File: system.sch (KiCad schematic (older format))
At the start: 38 parts, among them IC1 OSD335x, IC3 NAND_4GB, U8 SN74LVC1G06DCK, U9 74LVC1G07DCK, Y1 24MHz, Y2 32.768kHz

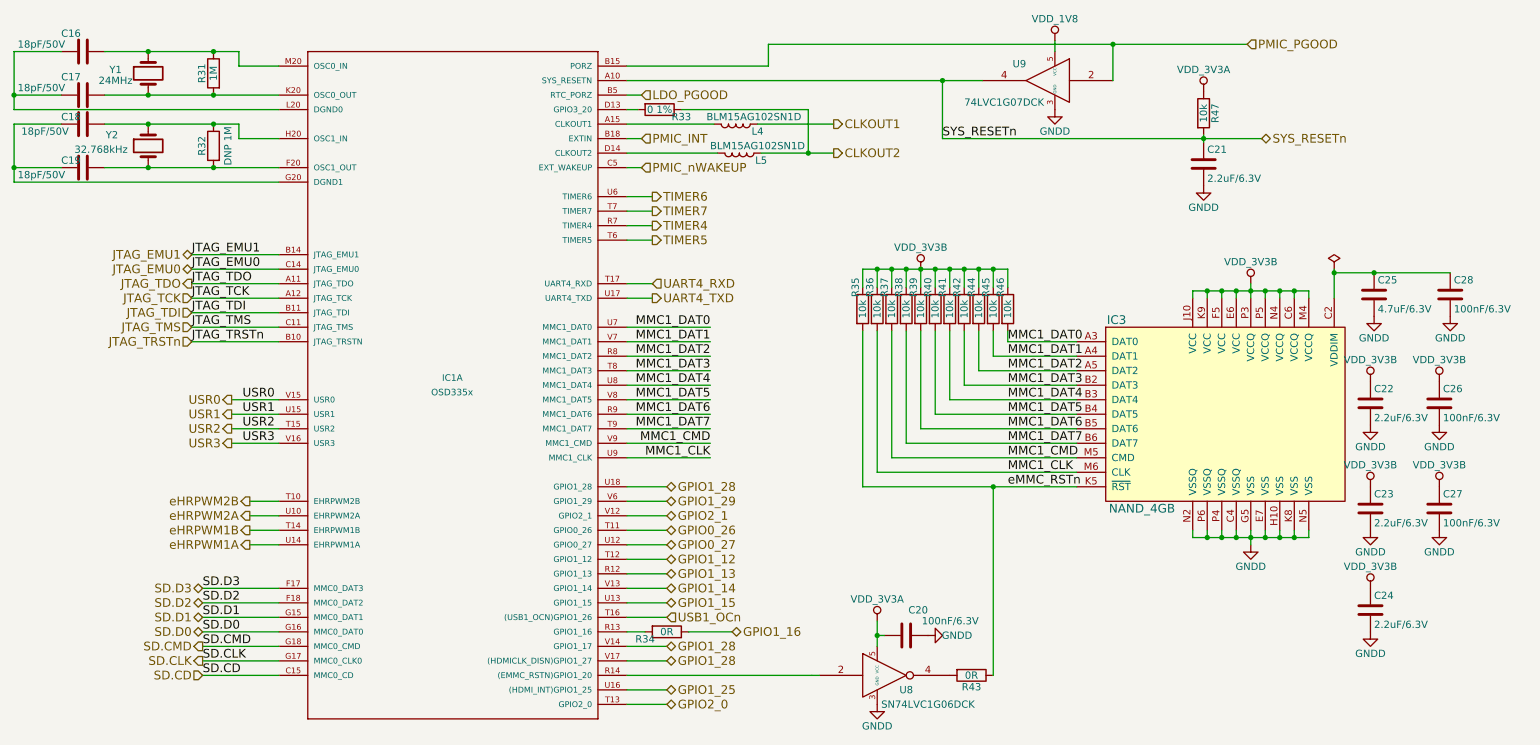
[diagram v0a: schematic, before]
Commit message: wip erc
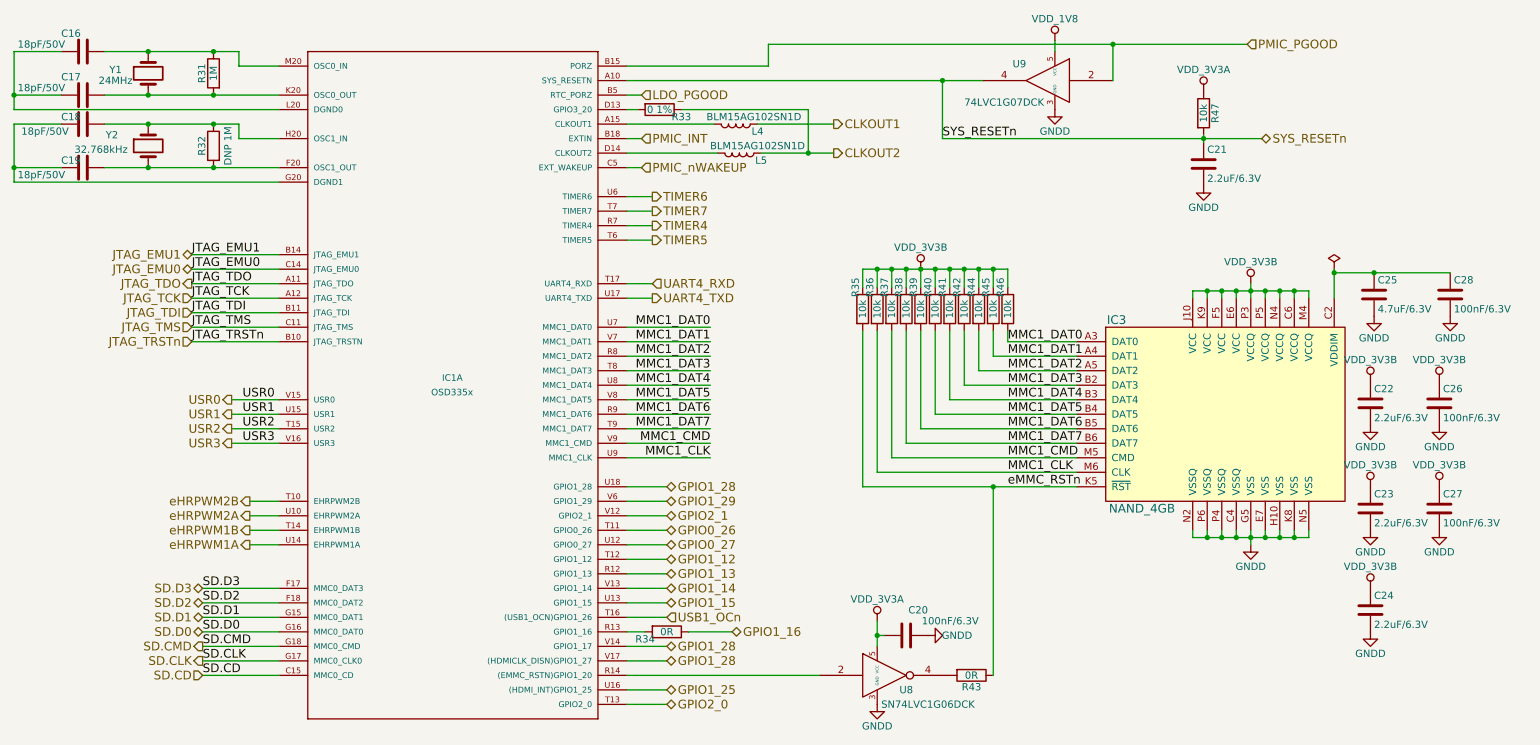
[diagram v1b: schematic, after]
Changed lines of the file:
@@
 $EndComp
 Wire Wire Line
-	1375 775  1675 775
-Wire Wire Line
-	1675 775  2125 775
-Wire Wire Line
-	2125 775  2300 775
-Wire Wire Line
-	1375 1075 1675 1075
-Wire Wire Line
-	1675 1075 2125 1075
-Wire Wire Line
-	2125 1075 2575 1075
+	1375 775  2300 775
+Wire Wire Line
+	1375 1075 2575 1075
 $Comp
 L R R31
@@
 	1075 775  750  775
 Wire Wire Line
-	750  775  750  1075
-Wire Wire Line
-	750  1075 750  1175
+	750  775  750  1175
 Wire Wire Line
 	750  1075 1075 1075
@@
 $EndComp
 Wire Wire Line
-	5950 725  8325 725
-Wire Wire Line
-	8325 725  9250 725
+	5950 725  9250 725
 Text HLabel 9250 725  2    60   Input ~ 0
 PMIC_PGOOD
@@
 $EndComp
 Wire Wire Line
-	4975 975  7150 975
-Wire Wire Line
-	7150 975  7425 975
+	4975 975  7425 975
 $Comp
 L GNDD #PWR75
@@
 Connection ~ 8325 725
 Wire Wire Line
-	7150 1375 8950 1375
-Wire Wire Line
-	8950 1375 9350 1375
+	7150 1375 9350 1375
 Wire Wire Line
 	7150 1375 7150 975
@@
 $EndComp
 Wire Wire Line
-	8950 1350 8950 1375
-Wire Wire Line
-	8950 1375 8950 1400
+	8950 1350 8950 1400
 Connection ~ 8950 1375
 $Comp
@@
 CLKOUT2
 Wire Wire Line
-	5900 1475 6225 1475
-Wire Wire Line
-	6225 1475 6400 1475
+	5900 1475 6400 1475
 $Comp
 L OSD335x IC1
@@
 $EndComp
 Wire Wire Line
-	1375 1275 1675 1275
-Wire Wire Line
-	1675 1275 2125 1275
-Wire Wire Line
-	2125 1275 2300 1275
-Wire Wire Line
-	1375 1575 1675 1575
-Wire Wire Line
-	1675 1575 2125 1575
-Wire Wire Line
-	2125 1575 2575 1575
+	1375 1275 2300 1275
+Wire Wire Line
+	1375 1575 2575 1575
 $Comp
 L R R32
@@
 	1075 1275 750  1275
 Wire Wire Line
-	750  1275 750  1575
-Wire Wire Line
-	750  1575 750  1675
+	750  1275 750  1675
 Wire Wire Line
 	750  1575 1075 1575
@@
 Connection ~ 9175 2425
 Wire Wire Line
-	9275 2375 9275 2425
-Wire Wire Line
-	9275 2425 9275 2475
+	9275 2375 9275 2475
 Connection ~ 9275 2425
 Wire Wire Line
@@
 	9675 2425 9675 2475
 Wire Wire Line
-	8875 2425 8975 2425
-Wire Wire Line
-	8975 2425 9075 2425
-Wire Wire Line
-	9075 2425 9175 2425
-Wire Wire Line
-	9175 2425 9275 2425
-Wire Wire Line
-	9275 2425 9375 2425
-Wire Wire Line
-	9375 2425 9475 2425
-Wire Wire Line
-	9475 2425 9575 2425
-Wire Wire Line
-	9575 2425 9675 2425
+	8875 2425 9675 2425
 $Comp
 L C C25
@@
 $EndComp
 Wire Wire Line
-	9850 2275 9850 2300
-Wire Wire Line
-	9850 2300 9850 2475
-Wire Wire Line
-	9850 2300 10125 2300
-Wire Wire Line
-	10125 2300 10650 2300
+	9850 2275 9850 2475
+Wire Wire Line
+	9850 2300 10650 2300
 $Comp
 L GNDD #PWR79
@@
 Connection ~ 9175 4125
 Wire Wire Line
-	9275 4075 9275 4125
-Wire Wire Line
-	9275 4125 9275 4175
+	9275 4075 9275 4175
 Connection ~ 9275 4125
 Wire Wire Line
@@
 	9675 4125 9675 4075
 Wire Wire Line
-	8875 4125 8975 4125
-Wire Wire Line
-	8975 4125 9075 4125
-Wire Wire Line
-	9075 4125 9175 4125
-Wire Wire Line
-	9175 4125 9275 4125
-Wire Wire Line
-	9275 4125 9375 4125
-Wire Wire Line
-	9375 4125 9475 4125
-Wire Wire Line
-	9475 4125 9575 4125
-Wire Wire Line
-	9575 4125 9675 4125
+	8875 4125 9675 4125
 $Comp
 L R R42
@@
 Connection ~ 6900 2275
 Wire Wire Line
-	6600 2275 6700 2275
-Wire Wire Line
-	6700 2275 6800 2275
-Wire Wire Line
-	6800 2275 6900 2275
-Wire Wire Line
-	6900 2275 7000 2275
-Wire Wire Line
-	7000 2275 7100 2275
-Wire Wire Line
-	7100 2275 7200 2275
-Wire Wire Line
-	7200 2275 7300 2275
-Wire Wire Line
-	7300 2275 7400 2275
-Wire Wire Line
-	7400 2275 7500 2275
-Wire Wire Line
-	7500 2275 7600 2275
+	6600 2275 7600 2275
 Wire Wire Line
 	7000 2275 7000 2400
@@
 	6600 2700 6600 3775
 Wire Wire Line
-	6600 3775 7500 3775
-Wire Wire Line
-	7500 3775 8075 3775
+	6600 3775 8075 3775
 Text Label 7600 2775 0    60   ~ 0
 MMC1_DAT0
@@
 	6750 4800 6700 4800
 Wire Wire Line
-	6700 4700 6700 4800
-Wire Wire Line
-	6700 4800 6700 4875
+	6700 4700 6700 4875
 Connection ~ 6700 4800
 Wire Wire Line
@@
 $EndComp
 Wire Wire Line
-	4975 5075 6250 5075
-Wire Wire Line
-	6250 5075 6250 5075
-Wire Wire Line
-	6250 5075 6300 5075
+	4975 5075 6300 5075
 Wire Wire Line
 	4975 3775 5250 3775

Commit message: erc passed
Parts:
- IC1: symbol OSD335x -> OSD335x-RESCUE-mateboard
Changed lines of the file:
@@
 	4975 975  7425 975
 $Comp
-L GNDD #PWR75
+L GNDD #PWR0106
 U 1 1 58AFE459
 P 7925 1175
-F 0 "#PWR75" H 7925 925 50  0001 C CNN
+F 0 "#PWR0106" H 7925 925 50  0001 C CNN
 F 1 "GNDD" H 7925 1025 50  0000 C CNN
 F 2 "" H 7925 1175 50  0000 C CNN
@@
 Connection ~ 8950 1375
 $Comp
-L VDD_3V3A #PWR76
+L VDD_3V3A #PWR0107
 U 1 1 58AFF28A
 P 8950 1050
-F 0 "#PWR76" H 8950 900 50  0001 C CNN
+F 0 "#PWR0107" H 8950 900 50  0001 C CNN
 F 1 "VDD_3V3A" H 8950 1200 50  0000 C CNN
 F 2 "" H 8950 1050 50  0000 C CNN
@@
 $EndComp
 $Comp
-L GNDD #PWR77
+L GNDD #PWR0108
 U 1 1 58AFF2DD
 P 8950 1700
-F 0 "#PWR77" H 8950 1450 50  0001 C CNN
+F 0 "#PWR0108" H 8950 1450 50  0001 C CNN
 F 1 "GNDD" H 8950 1550 50  0000 C CNN
 F 2 "" H 8950 1700 50  0000 C CNN
@@
 	5900 1475 6400 1475
 $Comp
-L OSD335x IC1
+L OSD335x-RESCUE-mateboard IC1
 U 1 1 58D2CE56
 P 3775 3075
+AR Path="/58D2CE56" Ref="IC1"  Part="1"
+AR Path="/58AC1B74/58D2CE56" Ref="IC1"  Part="1"
 F 0 "IC1" H 3700 3100 45  0000 L BNN
 F 1 "OSD335x" H 3625 3000 45  0000 L BNN
@@
 $EndComp
 $Comp
-L VDD_3V3B #PWR78
+L VDD_3V3B #PWR0109
 U 1 1 58D48CDC
 P 9275 2375
-F 0 "#PWR78" H 9275 2225 50  0001 C CNN
+F 0 "#PWR0109" H 9275 2225 50  0001 C CNN
 F 1 "VDD_3V3B" H 9275 2525 50  0000 C CNN
 F 2 "" H 9275 2375 50  0000 C CNN
@@
 $EndComp
 $Comp
-L GNDD #PWR86
+L GNDD #PWR0110
 U 1 1 58D48CFA
 P 10125 2600
-F 0 "#PWR86" H 10125 2350 50  0001 C CNN
+F 0 "#PWR0110" H 10125 2350 50  0001 C CNN
 F 1 "GNDD" H 10125 2450 50  0000 C CNN
 F 2 "" H 10125 2600 50  0000 C CNN
@@
 	9850 2300 10650 2300
 $Comp
-L GNDD #PWR79
+L GNDD #PWR0111
 U 1 1 58D48D02
 P 9275 4175
-F 0 "#PWR79" H 9275 3925 50  0001 C CNN
+F 0 "#PWR0111" H 9275 3925 50  0001 C CNN
 F 1 "GNDD" H 9275 4025 50  0000 C CNN
 F 2 "" H 9275 4175 50  0000 C CNN
@@
 $EndComp
 $Comp
-L VDD_3V3B #PWR72
+L VDD_3V3B #PWR0112
 U 1 1 58D48D66
 P 7000 2275
-F 0 "#PWR72" H 7000 2125 50  0001 C CNN
+F 0 "#PWR0112" H 7000 2125 50  0001 C CNN
 F 1 "VDD_3V3B" H 7000 2425 50  0000 C CNN
 F 2 "" H 7000 2275 50  0000 C CNN
@@
 $EndComp
 $Comp
-L VDD_3V3A #PWR70
+L VDD_3V3A #PWR0113
 U 1 1 58D48DB0
 P 6700 4700
-F 0 "#PWR70" H 6700 4550 50  0001 C CNN
+F 0 "#PWR0113" H 6700 4550 50  0001 C CNN
 F 1 "VDD_3V3A" H 6700 4850 50  0000 C CNN
 F 2 "" H 6700 4700 50  0000 C CNN
@@
 $EndComp
 $Comp
-L GNDD #PWR71
+L GNDD #PWR0114
 U 1 1 58D48DB6
 P 6700 5275
-F 0 "#PWR71" H 6700 5025 50  0001 C CNN
+F 0 "#PWR0114" H 6700 5025 50  0001 C CNN
 F 1 "GNDD" H 6700 5125 50  0000 C CNN
 F 2 "" H 6700 5275 50  0000 C CNN
@@
 $EndComp
 $Comp
-L GNDD #PWR73
+L GNDD #PWR0115
 U 1 1 58D48DC3
 P 7050 4800
-F 0 "#PWR73" H 7050 4550 50  0001 C CNN
+F 0 "#PWR0115" H 7050 4550 50  0001 C CNN
 F 1 "GNDD" V 7050 4600 50  0000 C CNN
 F 2 "" H 7050 4800 50  0000 C CNN
@@
 Connection ~ 7500 3775
 $Comp
-L PWR_FLAG #FLG3
+L PWR_FLAG #FLG0116
 U 1 1 58D48DD0
 P 9850 2275
-F 0 "#FLG3" H 9850 2350 50  0001 C CNN
+F 0 "#FLG0116" H 9850 2350 50  0001 C CNN
 F 1 "PWR_FLAG" H 9850 2425 50  0001 C CNN
 F 2 "" H 9850 2275 50  0001 C CNN
@@
 	5950 875  4975 875
 $Comp
-L VDD_1V8 #PWR74
+L VDD_1V8 #PWR0117
 U 1 1 58DA59D5
 P 7925 700
-F 0 "#PWR74" H 7925 550 50  0001 C CNN
+F 0 "#PWR0117" H 7925 550 50  0001 C CNN
 F 1 "VDD_1V8" H 7925 850 50  0000 C CNN
 F 2 "" H 7925 700 50  0000 C CNN
@@
 $EndComp
 $Comp
-L GNDD #PWR91
+L GNDD #PWR0118
 U 1 1 58DADD35
 P 10650 2600
-F 0 "#PWR91" H 10650 2350 50  0001 C CNN
+F 0 "#PWR0118" H 10650 2350 50  0001 C CNN
 F 1 "GNDD" H 10650 2450 50  0000 C CNN
 F 2 "" H 10650 2600 50  0000 C CNN
@@
 $EndComp
 $Comp
-L GNDD #PWR81
+L GNDD #PWR0119
 U 1 1 58DAEBBD
 P 10100 3350
-F 0 "#PWR81" H 10100 3100 50  0001 C CNN
+F 0 "#PWR0119" H 10100 3100 50  0001 C CNN
 F 1 "GNDD" H 10100 3200 50  0000 C CNN
 F 2 "" H 10100 3350 50  0000 C CNN
@@
 $EndComp
 $Comp
-L GNDD #PWR88
+L GNDD #PWR0120
 U 1 1 58DAEC64
 P 10575 3350
-F 0 "#PWR88" H 10575 3100 50  0001 C CNN
+F 0 "#PWR0120" H 10575 3100 50  0001 C CNN
 F 1 "GNDD" H 10575 3200 50  0000 C CNN
 F 2 "" H 10575 3350 50  0000 C CNN
@@
 	5400 4775 5700 4775
 $Comp
-L VDD_3V3B #PWR80
+L VDD_3V3B #PWR0121
 U 1 1 58DB0C91
 P 10100 3050
-F 0 "#PWR80" H 10100 2900 50  0001 C CNN
+F 0 "#PWR0121" H 10100 2900 50  0001 C CNN
 F 1 "VDD_3V3B" H 10100 3200 50  0000 C CNN
 F 2 "" H 10100 3050 50  0000 C CNN
@@
 $EndComp
 $Comp
-L VDD_3V3B #PWR87
+L VDD_3V3B #PWR0122
 U 1 1 58DB0D28
 P 10575 3050
-F 0 "#PWR87" H 10575 2900 50  0001 C CNN
+F 0 "#PWR0122" H 10575 2900 50  0001 C CNN
 F 1 "VDD_3V3B" H 10575 3200 50  0000 C CNN
 F 2 "" H 10575 3050 50  0000 C CNN
@@
 $EndComp
 $Comp
-L GNDD #PWR83
+L GNDD #PWR0123
 U 1 1 58DB0E3C
 P 10100 4075
-F 0 "#PWR83" H 10100 3825 50  0001 C CNN
+F 0 "#PWR0123" H 10100 3825 50  0001 C CNN
 F 1 "GNDD" H 10100 3925 50  0000 C CNN
 F 2 "" H 10100 4075 50  0000 C CNN
@@
 $EndComp
 $Comp
-L VDD_3V3B #PWR82
+L VDD_3V3B #PWR0124
 U 1 1 58DB0E42
 P 10100 3775
-F 0 "#PWR82" H 10100 3625 50  0001 C CNN
+F 0 "#PWR0124" H 10100 3625 50  0001 C CNN
 F 1 "VDD_3V3B" H 10100 3925 50  0000 C CNN
 F 2 "" H 10100 3775 50  0000 C CNN
@@
 $EndComp
 $Comp
-L GNDD #PWR85
+L GNDD #PWR0125
 U 1 1 58DB0EE7
 P 10100 4775
-F 0 "#PWR85" H 10100 4525 50  0001 C CNN
+F 0 "#PWR0125" H 10100 4525 50  0001 C CNN
 F 1 "GNDD" H 10100 4625 50  0000 C CNN
 F 2 "" H 10100 4775 50  0000 C CNN
@@
 $EndComp
 $Comp
-L VDD_3V3B #PWR84
+L VDD_3V3B #PWR0126
 U 1 1 58DB0EED
 P 10100 4475
-F 0 "#PWR84" H 10100 4325 50  0001 C CNN
+F 0 "#PWR0126" H 10100 4325 50  0001 C CNN
 F 1 "VDD_3V3B" H 10100 4625 50  0000 C CNN
 F 2 "" H 10100 4475 50  0000 C CNN
@@
 $EndComp
 $Comp
-L GNDD #PWR90
+L GNDD #PWR0127
 U 1 1 58DB11F2
 P 10575 4075
-F 0 "#PWR90" H 10575 3825 50  0001 C CNN
+F 0 "#PWR0127" H 10575 3825 50  0001 C CNN
 F 1 "GNDD" H 10575 3925 50  0000 C CNN
 F 2 "" H 10575 4075 50  0000 C CNN
@@
 $EndComp
 $Comp
-L VDD_3V3B #PWR89
+L VDD_3V3B #PWR0128
 U 1 1 58DB11F8
 P 10575 3775
-F 0 "#PWR89" H 10575 3625 50  0001 C CNN
+F 0 "#PWR0128" H 10575 3625 50  0001 C CNN
 F 1 "VDD_3V3B" H 10575 3925 50  0000 C CNN
 F 2 "" H 10575 3775 50  0000 C CNN
